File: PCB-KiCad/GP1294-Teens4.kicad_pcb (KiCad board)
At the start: 2 copper layers, 178.5 x 99.9 mm, 37 parts, among them IC1 74132D, IC2 XL6009, IC3 ZXBM5210, SW1 SW_Push, SW2 SW_Push, SW3 SW_Push, SW4 SW_Push, SW5 SW_Push, U3 R-78B5.0-2.0

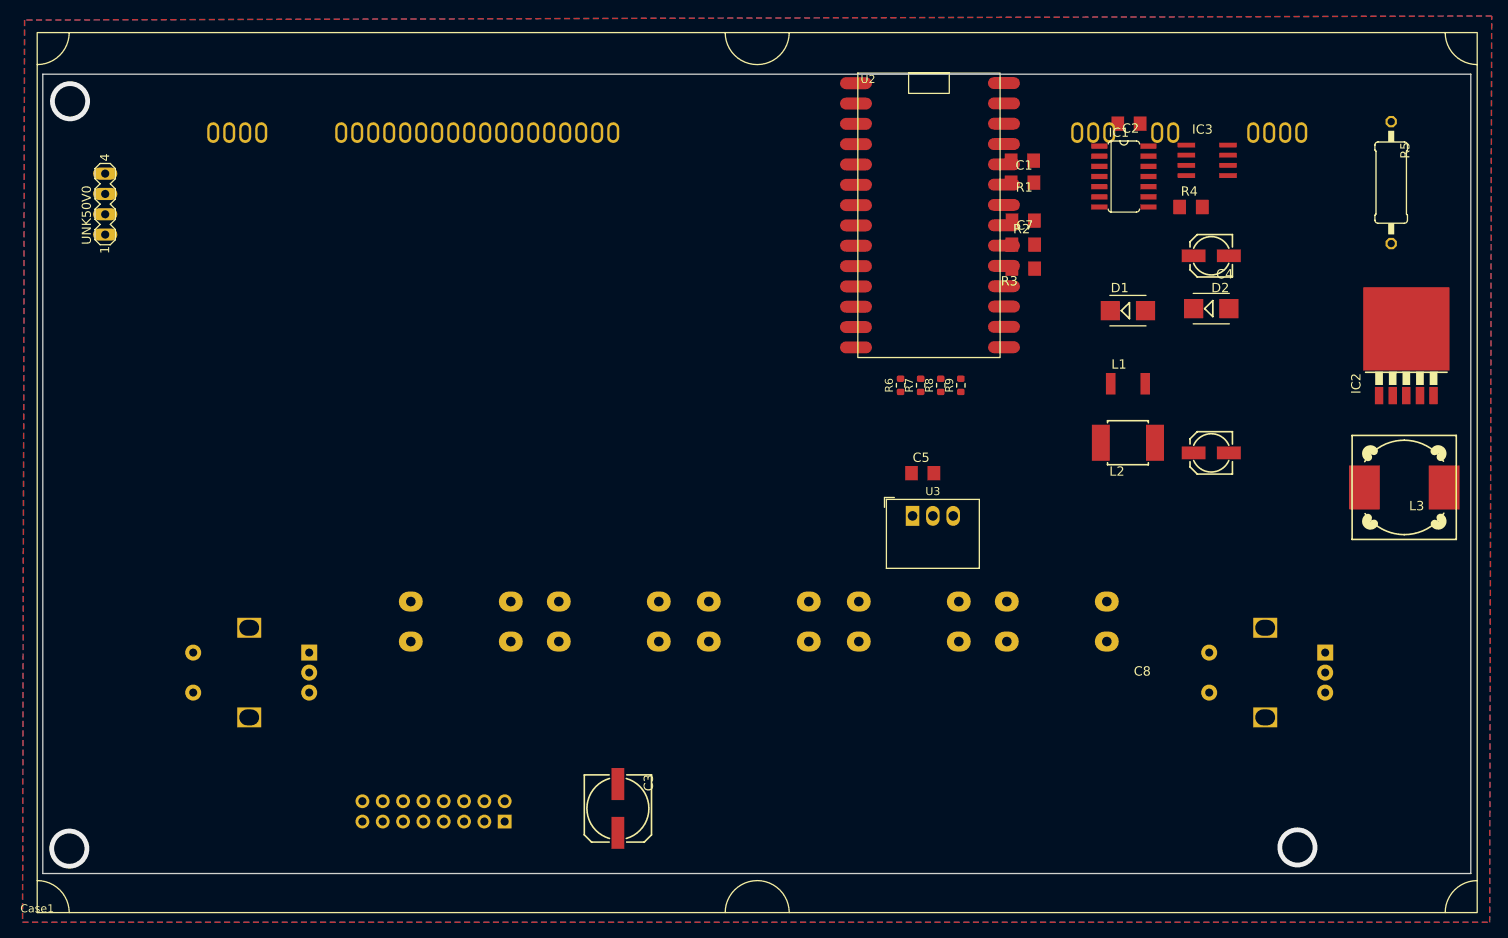
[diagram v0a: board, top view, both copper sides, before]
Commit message: GP12.. better case and stuff
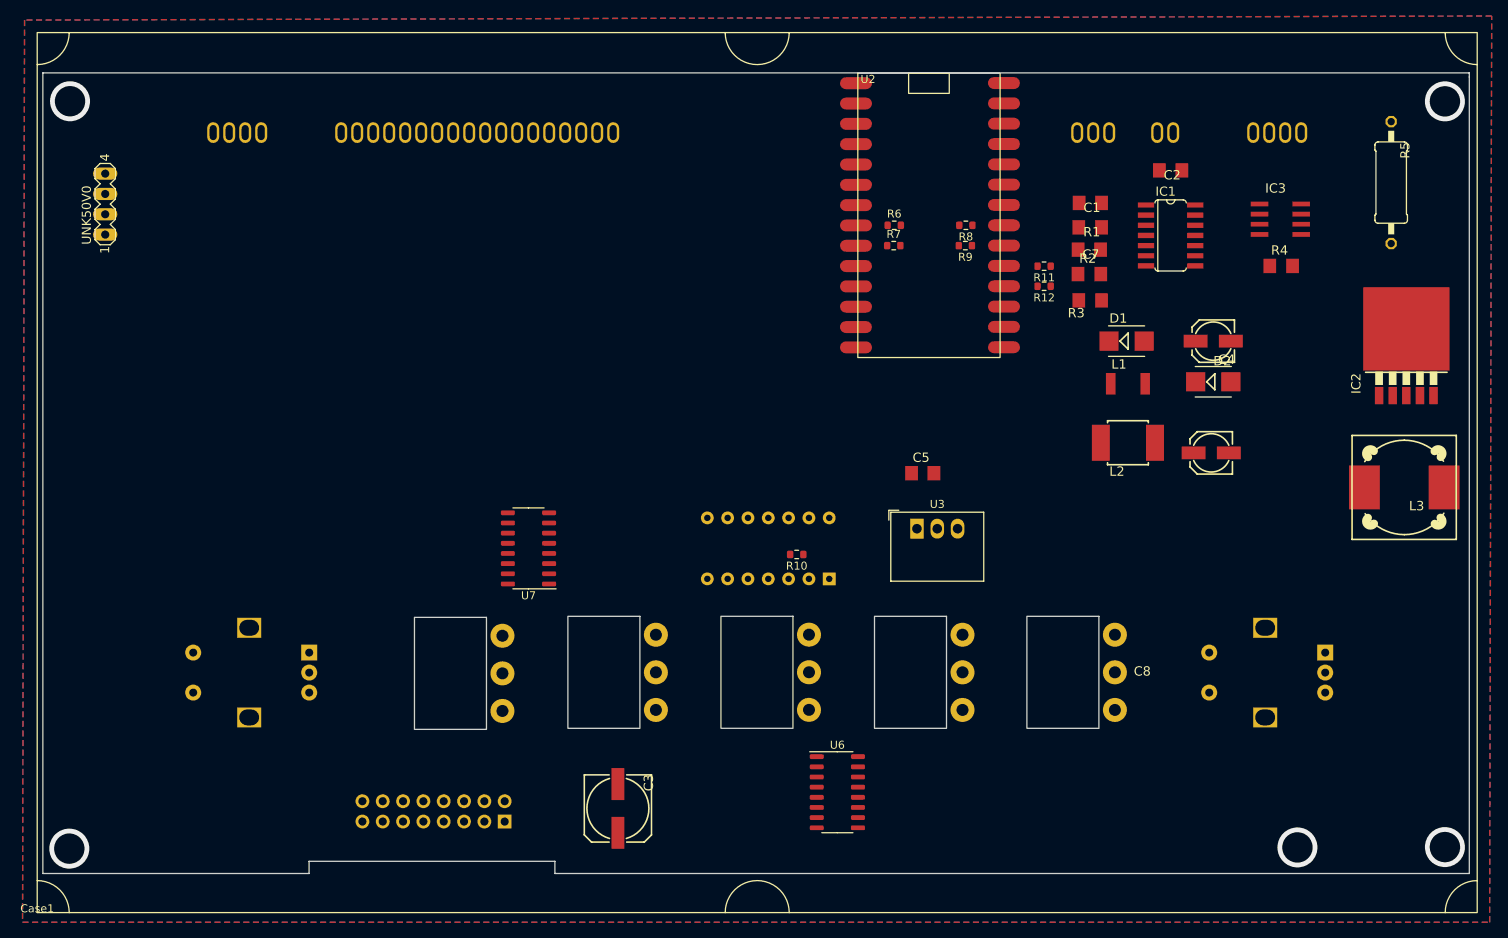
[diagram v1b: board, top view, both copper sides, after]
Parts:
- added R10: 100, Resistor_SMD:R_0603_1608Metric, F.Cu at (154.9, 110.2)
- added R11: 10k, Resistor_SMD:R_0603_1608Metric, F.Cu at (185.9, 74.2)
- added R12: 10k, Resistor_SMD:R_0603_1608Metric, F.Cu at (185.9, 76.7)
- added U5: ATtiny84A-P, Package_DIP:DIP-14_W7.62mm, B.Cu at (159.0, 113.3)
- added U6: 74HC165, Package_SO:SO-16_3.9x9.9mm_P1.27mm, F.Cu at (160.0, 140.0)
- added U7: 74HC165, Package_SO:SO-16_3.9x9.9mm_P1.27mm, F.Cu at (121.4, 109.5)
- SW1, SW2, SW3, SW4, SW5: value SW_Push -> SW_DPDT_x2; footprint Button_Switch_THT:SW_PUSH-12mm_Wuerth-430476085716 -> VFDs-Library:SwitchMS500Ecut
- moved SW5 82.5 mm to (111.7, 125.1)
- moved SW1 69.6 mm to (188.2, 125.0)
- moved SW4 45.2 mm to (130.8, 125.0)
- moved SW2 32.7 mm to (169.2, 125.0)
- moved R8 20.2 mm to (176.1, 69.1), turned to 180 degrees
- moved R6 20.0 mm to (167.1, 69.1), turned to 0 degrees
- moved R7 17.8 mm to (167.1, 71.6), turned to 0 degrees
- moved R9 17.5 mm to (176.0, 71.6), turned to 180 degrees
- moved R4 13.5 mm to (215.5, 74.2)
- moved IC3 11.7 mm to (215.4, 68.3)
- moved SW3 11.0 mm to (150.0, 125.0)
- moved C4 10.7 mm to (207.0, 83.6)
- moved R1 10.1 mm to (191.6, 69.3)
- moved C1 10.0 mm to (191.6, 66.3)
- moved IC1 9.40 mm to (201.7, 70.4)
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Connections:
- ENC1 pad A: unconnected-(ENC1-PadA) -> /inputs/enc1a
- ENC1 pad B: unconnected-(ENC1-PadB) -> /inputs/enc1b
- ENC1 pad C: unconnected-(ENC1-PadC) -> GND
- ENC1 pad S1: unconnected-(ENC1-PadS1) -> /inputs/enc1c
- ENC1 pad S2: unconnected-(ENC1-PadS2) -> GND
- ENC2 pad A: unconnected-(ENC2-PadA) -> /inputs/enc2a
- ENC2 pad B: unconnected-(ENC2-PadB) -> /inputs/enc2b
- ENC2 pad C: unconnected-(ENC2-PadC) -> GND
- ENC2 pad S1: unconnected-(ENC2-PadS1) -> /inputs/enc2c
- ENC2 pad S2: unconnected-(ENC2-PadS2) -> GND
- SW1 pad 1: GND -> Net-(SW1A-A)
- SW1 pad 2: Net-(U2-5) -> GND
- SW2 pad 1: unconnected-(SW2-Pad1) -> Net-(SW2A-A)
- SW2 pad 2: unconnected-(SW2-Pad2) -> GND
- SW3 pad 1: GND -> Net-(SW3A-A)
- SW3 pad 2: Net-(U2-3) -> GND
- SW4 pad 1: GND -> Net-(SW4A-A)
- SW4 pad 2: Net-(U2-4) -> GND
- SW5 pad 1: unconnected-(SW5-Pad1) -> Net-(SW5A-A)
- SW5 pad 2: unconnected-(SW5-Pad2) -> GND
- U2 pad 18: unconnected-(U2-A2-Pad18) -> /SDA
- U2 pad 19: unconnected-(U2-A3-Pad19) -> /SCL
- U2 pad 5: Net-(U2-3) -> unconnected-(U2-3-Pad5)
- U2 pad 6: Net-(U2-4) -> unconnected-(U2-4-Pad6)
- U2 pad 7: Net-(U2-5) -> unconnected-(U2-5-Pad7)
- U4 pad 11: unconnected-(U4-SDA-Pad11) -> /SDA
- U4 pad 13: unconnected-(U4-SCL-Pad13) -> /SCL
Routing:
- net GND: vias 3 -> 5
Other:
- board size 178.5 x 99.9 mm -> 178.3 x 100.1 mm
